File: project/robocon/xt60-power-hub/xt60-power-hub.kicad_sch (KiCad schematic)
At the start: 12 parts, among them J1 IN, J2 OUT1, J3 OUT2, J4 OUT3, J5 OUT4, J6 OUT5

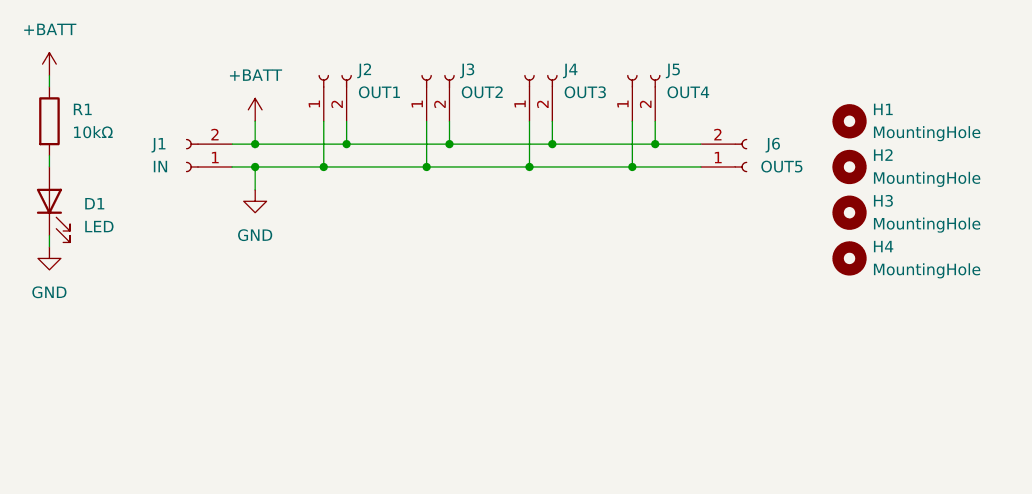
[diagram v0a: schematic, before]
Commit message: 2026/07/15/10:30
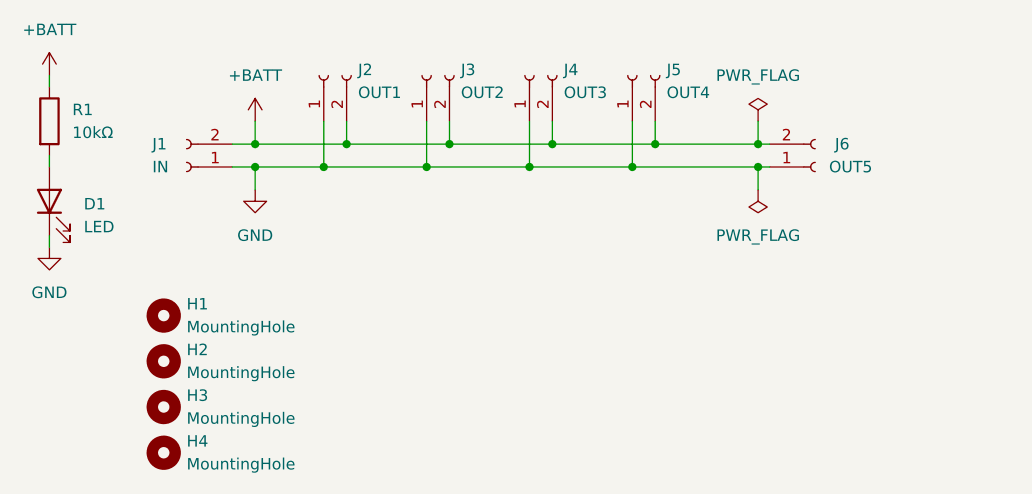
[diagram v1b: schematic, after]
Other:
- moved on the sheet: H1, H2, H3, H4, J6

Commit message: 2026/07/16/09:30
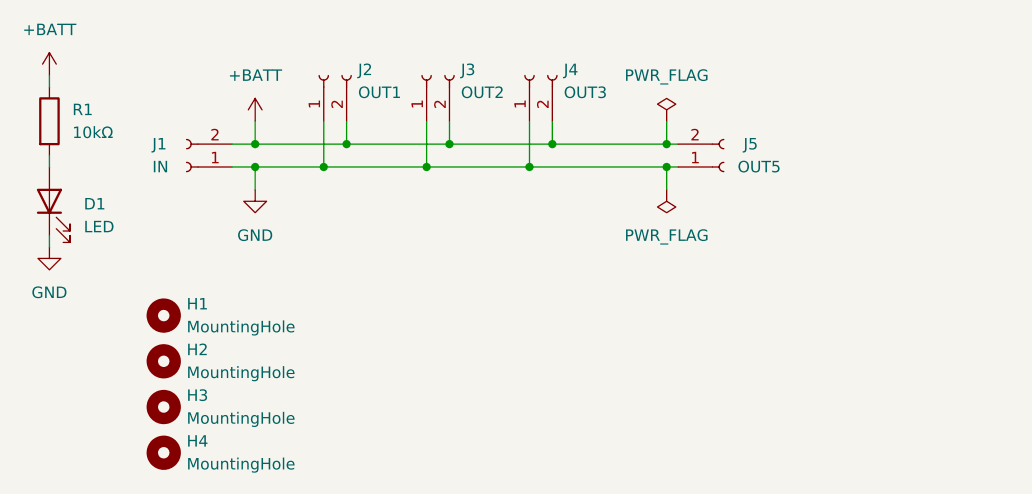
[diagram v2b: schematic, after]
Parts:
- removed J5: OUT4, Connector_AMASS:AMASS_XT60PW-F_1x02_P7.20mm_Horizontal, symbol Connector:Conn_01x02_Socket
- renumbered J6 to J5
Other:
- moved on the sheet: J5
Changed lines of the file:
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@@
 	(paper "A4")
 	(junction
-		(at 182.88 80.01)
+		(at 151.13 77.47)
+		(diameter 0)
+		(color 0 0 0 0)
+	)
+	(junction
+		(at 140.97 80.01)
+		(diameter 0)
+		(color 0 0 0 0)
+	)
+	(junction
+		(at 160.02 80.01)
+		(diameter 0)
+		(color 0 0 0 0)
+	)
+	(junction
+		(at 140.97 77.47)
+		(diameter 0)
+		(color 0 0 0 0)
+	)
+	(junction
+		(at 173.99 77.47)
+		(diameter 0)
+		(color 0 0 0 0)
+	)
+	(junction
+		(at 186.69 80.01)
+		(diameter 0)
+		(color 0 0 0 0)
+	)
+	(junction
+		(at 186.69 77.47)
+		(diameter 0)
+		(color 0 0 0 0)
+	)
+	(junction
+		(at 148.59 80.01)
+		(diameter 0)
+		(color 0 0 0 0)
+	)
+	(junction
+		(at 162.56 77.47)
 		(diameter 0)
 		(color 0 0 0 0)
@@
 		(color 0 0 0 0)
 	)
-	(junction
-		(at 185.42 77.47)
-		(diameter 0)
-		(color 0 0 0 0)
-	)
-	(junction
-		(at 151.13 77.47)
-		(diameter 0)
-		(color 0 0 0 0)
-	)
-	(junction
-		(at 140.97 80.01)
-		(diameter 0)
-		(color 0 0 0 0)
-	)
-	(junction
-		(at 160.02 80.01)
-		(diameter 0)
-		(color 0 0 0 0)
-	)
-	(junction
-		(at 140.97 77.47)
-		(diameter 0)
-		(color 0 0 0 0)
-	)
-	(junction
-		(at 196.85 80.01)
-		(diameter 0)
-		(color 0 0 0 0)
-	)
-	(junction
-		(at 196.85 77.47)
-		(diameter 0)
-		(color 0 0 0 0)
-	)
-	(junction
-		(at 148.59 80.01)
-		(diameter 0)
-		(color 0 0 0 0)
-	)
-	(junction
-		(at 162.56 77.47)
-		(diameter 0)
-		(color 0 0 0 0)
-	)
-	(junction
-		(at 173.99 77.47)
-		(diameter 0)
-		(color 0 0 0 0)
-	)
 	(wire
 		(pts
@@
 	(wire
 		(pts
-			(xy 196.85 74.93) (xy 196.85 77.47)
+			(xy 186.69 74.93) (xy 186.69 77.47)
 		)
 		(stroke
@@
 	(wire
 		(pts
-			(xy 182.88 80.01) (xy 171.45 80.01)
+			(xy 171.45 80.01) (xy 186.69 80.01)
 		)
 		(stroke
@@
 	(wire
 		(pts
-			(xy 198.12 80.01) (xy 196.85 80.01)
+			(xy 187.96 80.01) (xy 186.69 80.01)
 		)
 		(stroke
@@
 	(wire
 		(pts
-			(xy 196.85 80.01) (xy 196.85 82.55)
-		)
-		(stroke
-			(width 0)
-			(type default)
-		)
-	)
-	(wire
-		(pts
-			(xy 185.42 74.93) (xy 185.42 77.47)
-		)
-		(stroke
-			(width 0)
-			(type default)
-		)
-	)
-	(wire
-		(pts
-			(xy 198.12 77.47) (xy 196.85 77.47)
+			(xy 186.69 80.01) (xy 186.69 82.55)
+		)
+		(stroke
+			(width 0)
+			(type default)
+		)
+	)
+	(wire
+		(pts
+			(xy 187.96 77.47) (xy 186.69 77.47)
 		)
 		(stroke
@@
 	(wire
 		(pts
-			(xy 185.42 77.47) (xy 173.99 77.47)
+			(xy 173.99 77.47) (xy 186.69 77.47)
 		)
 		(stroke
@@
 	(wire
 		(pts
-			(xy 182.88 74.93) (xy 182.88 80.01)
-		)
-		(stroke
-			(width 0)
-			(type default)
-		)
-	)
-	(wire
-		(pts
 			(xy 171.45 74.93) (xy 171.45 80.01)
 		)
@@
 		(pts
 			(xy 148.59 74.93) (xy 148.59 80.01)
-		)
-		(stroke
-			(width 0)
-			(type default)
-		)
-	)
-	(wire
-		(pts
-			(xy 196.85 77.47) (xy 185.42 77.47)
-		)
-		(stroke
-			(width 0)
-			(type default)
-		)
-	)
-	(wire
-		(pts
-			(xy 196.85 80.01) (xy 182.88 80.01)
 		)
 		(stroke
@@
 	(symbol
 		(lib_id "power:PWR_FLAG")
-		(at 196.85 82.55 180)
+		(at 186.69 82.55 180)
 		(unit 1)
 		(body_style 1)
@@
 		(fields_autoplaced yes)
 		(property "Reference" "#FLG02"
-			(at 196.85 84.455 0)
+			(at 186.69 84.455 0)
 			(hide yes)
 			(show_name no)
@@
 		)
 		(property "Value" "PWR_FLAG"
-			(at 196.85 87.63 0)
+			(at 186.69 87.63 0)
 			(show_name no)
 			(do_not_autoplace no)
@@
 		)
 		(property "Footprint" ""
-			(at 196.85 82.55 0)
+			(at 186.69 82.55 0)
 			(hide yes)
 			(show_name no)
@@
 		)
 		(property "Datasheet" ""
-			(at 196.85 82.55 0)
+			(at 186.69 82.55 0)
 			(hide yes)
 			(show_name no)
@@
 		)
 		(property "Description" "Special symbol for telling ERC where power comes from"
-			(at 196.85 82.55 0)
+			(at 186.69 82.55 0)
 			(hide yes)
 			(show_name no)
@@
 	(symbol
 		(lib_id "power:PWR_FLAG")
-		(at 196.85 74.93 0)
+		(at 186.69 74.93 0)
 		(unit 1)
 		(body_style 1)
@@
 		(fields_autoplaced yes)
 		(property "Reference" "#FLG01"
-			(at 196.85 73.025 0)
+			(at 186.69 73.025 0)
 			(hide yes)
 			(show_name no)
@@
 		)
 		(property "Value" "PWR_FLAG"
-			(at 196.85 69.85 0)
+			(at 186.69 69.85 0)
 			(show_name no)
 			(do_not_autoplace no)
@@
 		)
 		(property "Footprint" ""
-			(at 196.85 74.93 0)
+			(at 186.69 74.93 0)
 			(hide yes)
 			(show_name no)
@@
 		)
 		(property "Datasheet" ""
-			(at 196.85 74.93 0)
+			(at 186.69 74.93 0)
 			(hide yes)
 			(show_name no)
@@
 		)
 		(property "Description" "Special symbol for telling ERC where power comes from"
-			(at 196.85 74.93 0)
+			(at 186.69 74.93 0)
 			(hide yes)
 			(show_name no)
@@
 	(symbol
 		(lib_id "Connector:Conn_01x02_Socket")
-		(at 182.88 69.85 90)
-		(unit 1)
-		(body_style 1)
-		(exclude_from_sim no)
-		(in_bom yes)
-		(on_board yes)
-		(in_pos_files yes)
-		(dnp no)
-		(fields_autoplaced yes)
-		(property "Reference" "J5"
-			(at 186.69 69.2149 90)
-			(show_name no)
-			(do_not_autoplace no)
-			(effects
-				(font
-					(size 1.27 1.27)
-				)
-				(justify right)
-			)
-		)
-		(property "Value" "OUT4"
-			(at 186.69 71.7549 90)
-			(show_name no)
-			(do_not_autoplace no)
-			(effects
-				(font
-					(size 1.27 1.27)
-				)
-				(justify right)
-			)
-		)
-		(property "Footprint" "Connector_AMASS:AMASS_XT60PW-F_1x02_P7.20mm_Horizontal"
-			(at 182.88 69.85 0)
-			(hide yes)
-			(show_name no)
-			(do_not_autoplace no)
-			(effects
-				(font
-					(size 1.27 1.27)
-				)
-			)
-		)
-		(property "Datasheet" ""
-			(at 182.88 69.85 0)
-			(hide yes)
-			(show_name no)
-			(do_not_autoplace no)
-			(effects
-				(font
-					(size 1.27 1.27)
-				)
-			)
-		)
-		(property "Description" "Generic connector, single row, 01x02, script generated"
-			(at 182.88 69.85 0)
-			(hide yes)
-			(show_name no)
-			(do_not_autoplace no)
-			(effects
-				(font
-					(size 1.27 1.27)
-				)
-			)
-		)
-		(pin "1"
-		)
-		(pin "2"
-		)
-		(instances
-			(project "xt60-power-hub"
-				(path "/1ffc8a7d-446d-4d87-80cb-e72e4474d330"
-					(reference "J5")
-					(unit 1)
-				)
-			)
-		)
-	)
-	(symbol
-		(lib_id "Connector:Conn_01x02_Socket")
 		(at 171.45 69.85 90)
 		(unit 1)
@@
 	(symbol
 		(lib_id "Connector:Conn_01x02_Socket")
-		(at 203.2 80.01 0)
+		(at 193.04 80.01 0)
 		(mirror x)
 		(unit 1)
@@
 		(in_pos_files yes)
 		(dnp no)
-		(property "Reference" "J6"
-			(at 207.01 77.4699 0)
+		(property "Reference" "J5"
+			(at 196.85 77.4699 0)
 			(show_name no)
 			(do_not_autoplace no)
@@
 		)
 		(property "Value" "OUT5"
-			(at 209.55 80.01 0)
+			(at 199.39 80.01 0)
 			(show_name no)
 			(do_not_autoplace no)
@@
 		)
 		(property "Footprint" "Connector_AMASS:AMASS_XT60PW-F_1x02_P7.20mm_Horizontal"
-			(at 203.2 80.01 0)
+			(at 193.04 80.01 0)
 			(hide yes)
 			(show_name no)
@@
 		)
 		(property "Datasheet" ""
-			(at 203.2 80.01 0)
+			(at 193.04 80.01 0)
 			(hide yes)
 			(show_name no)
@@
 		)
 		(property "Description" "Generic connector, single row, 01x02, script generated"
-			(at 203.2 80.01 0)
+			(at 193.04 80.01 0)
 			(hide yes)
 			(show_name no)
@@
 			(project "xt60-power-hub"
 				(path "/1ffc8a7d-446d-4d87-80cb-e72e4474d330"
-					(reference "J6")
+					(reference "J5")
 					(unit 1)
 				)
